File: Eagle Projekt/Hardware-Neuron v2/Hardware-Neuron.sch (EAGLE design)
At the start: 58 parts, among them IC1 74LVC1G125DBV, IC10 74LVC1G125DBV, IC11 74LVC1G125DBV, IC12 74LVC1G125DBV, IC13 74AHC1G86DBV, IC14 74LVC1G125DBV, IC15 74LVC1G125DBV, IC16 74LVC1G125DBV, IC17 74LVC1G125DBV, IC18 74AHC1G14DCK, IC19 74LVC1G125DBV, IC2 74LVC1G125DBV, IC20 74LVC1G125DBV, IC21 74LVC1G125DBV, IC22 74LVC1G125DBV, IC3 74LVC1G125DBV, IC4 74LVC1G125DBV, IC5 74LVC1G125DBV, IC6 74LVC1G125DBV, IC7 74AUC1G06DBV, IC8 74AHC1G08DBV, IC9 74LVC1G125DBV, Q1 FDN360P, Q10 FDN360P, Q11 BSS123, Q2 FDN360P, Q3 FDN360P, Q4 FDN360P, Q5 FDN360P, Q6 FDN360P, Q7 FDN360P, Q8 FDN360P, Q9 FDN360P

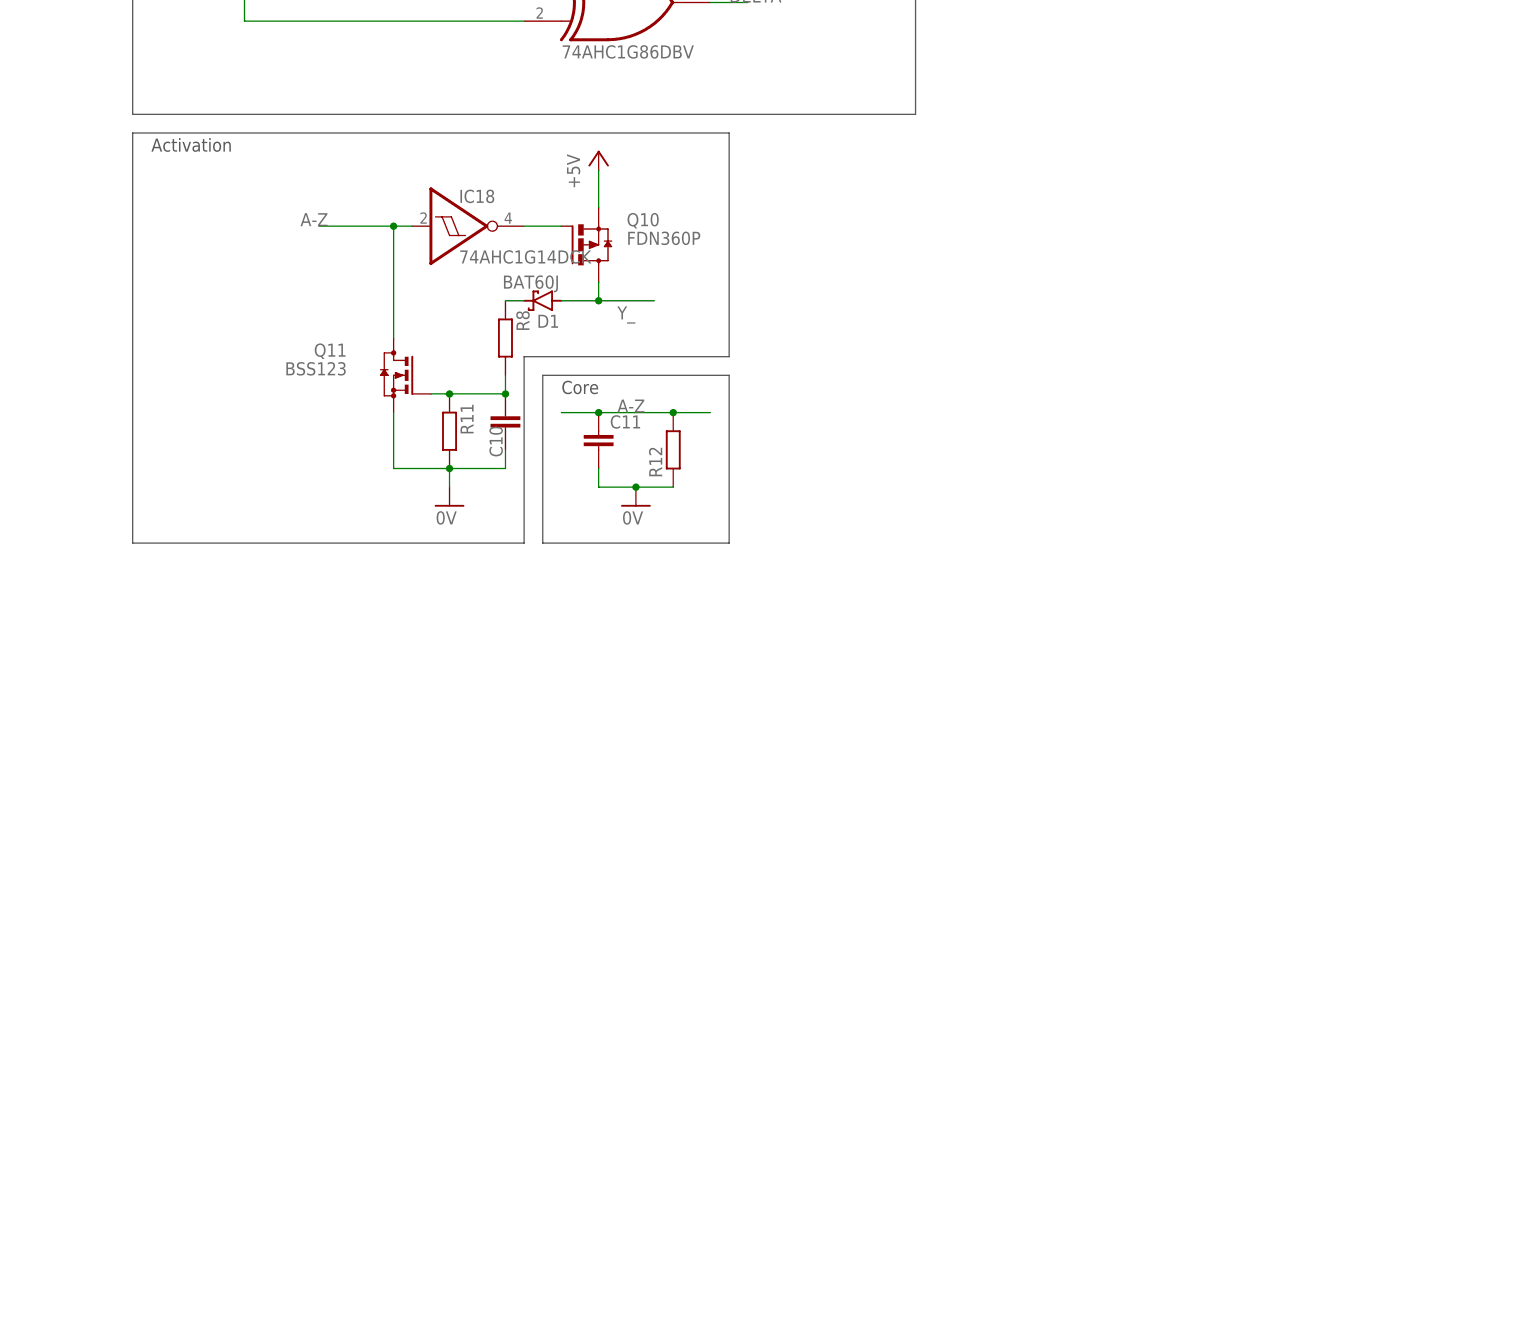
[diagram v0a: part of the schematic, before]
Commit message: malik aar und eagle
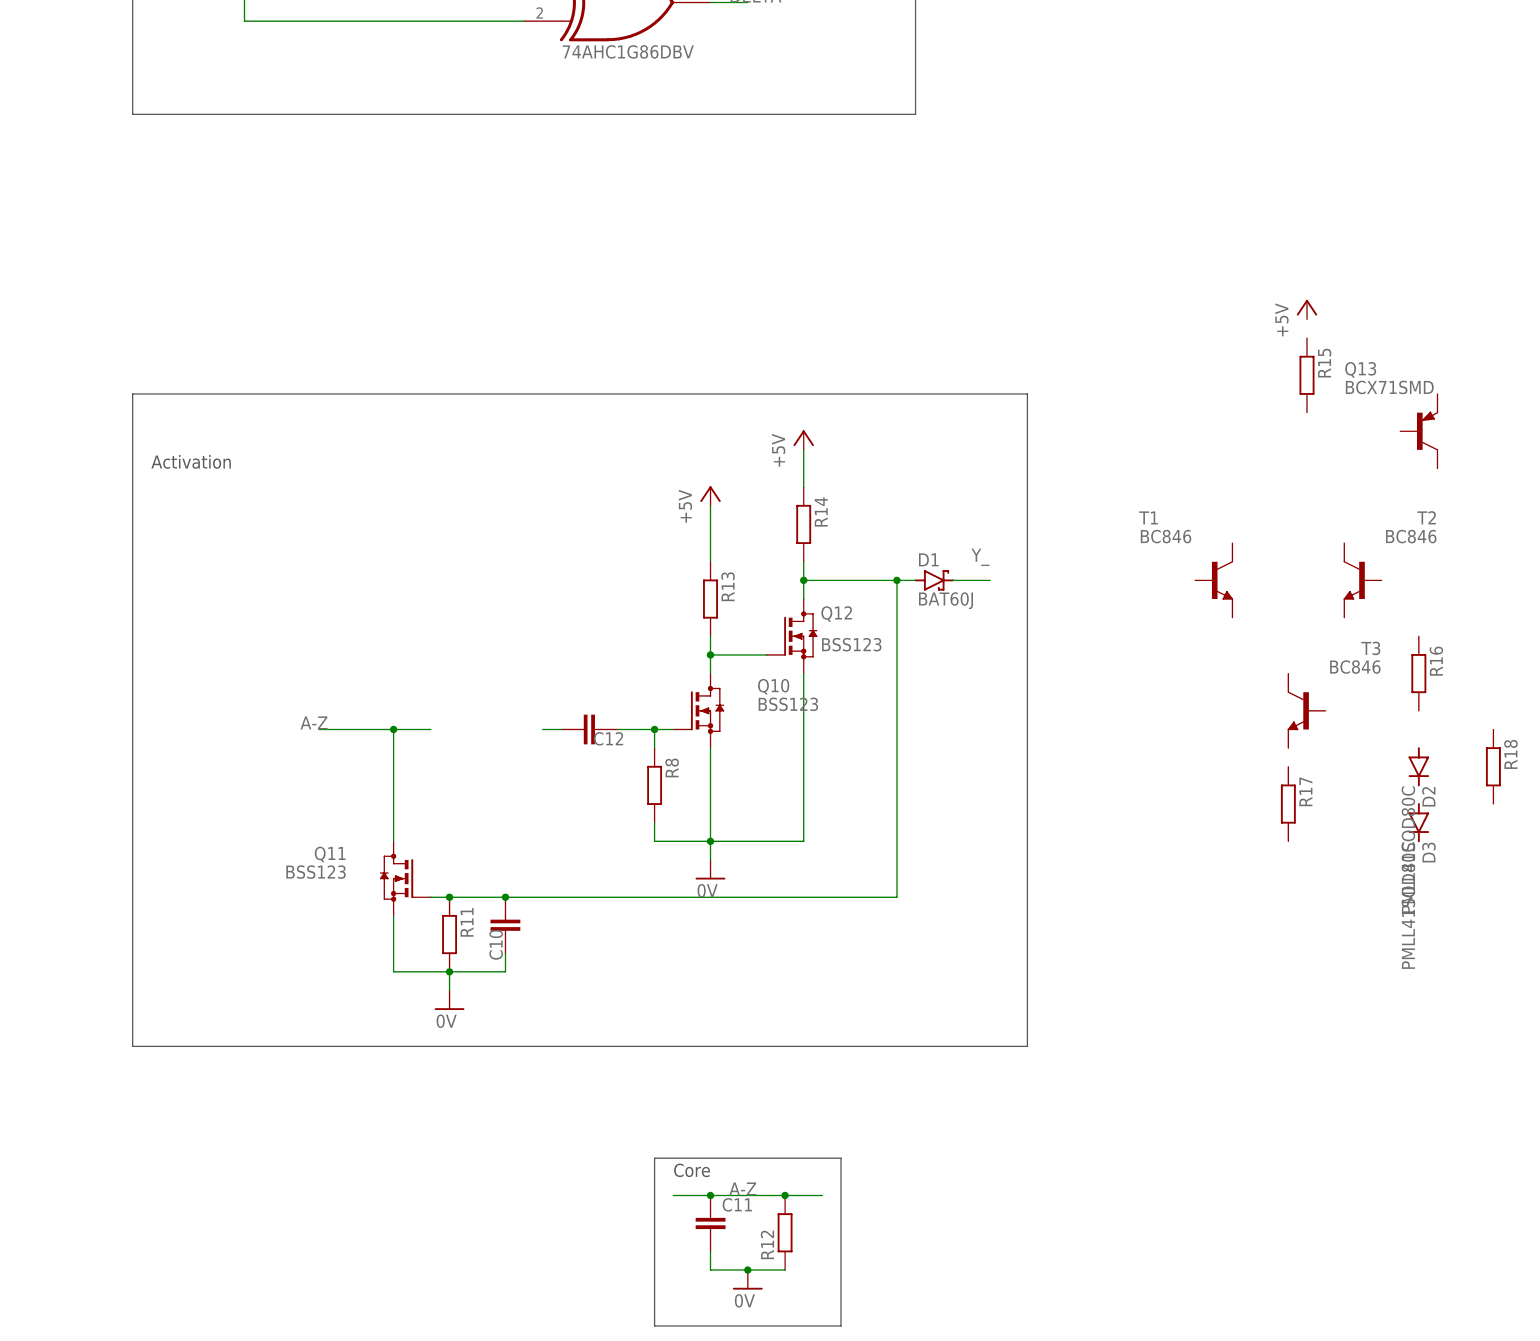
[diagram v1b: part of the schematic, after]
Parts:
- removed IC18: 74AHC1G14DCK, 74xx-little-de:74AHC1G14DCK
- added C12: (no value), rcl:C-EUC1206
- added D2, D3: PMLL41SOD80C, diode:PMLL41SOD80C
- added Q12: BSS123, transistor-small-signal:BSS123
- added Q13: BCX71SMD, transistor-pnp:BCX71SMD
- added R13, R14, R15, R16, R17, R18: (no value), rcl:R-EU_R1206
- added T1, T2, T3: BC846, transistor:BC846
- Q10: value FDN360P -> BSS123; device transistor-power:FDN360P -> transistor-small-signal:BSS123
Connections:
- new net N$3: C12.2, Q10.G, R8.1
- net +5V: now also R13.1, R14.1; no longer Q10.S
- net 0V: now also Q10.S, Q12.S, R8.2
- net A-Z: no longer IC18A.I
- net N$4: now also D1.A, Q12.D, R14.2; no longer R8.2
- net N$5: now also Q10.D, Q12.G, R13.2; no longer D1.C, R8.1
- net N$7: now also C12.1; no longer IC18A.O, Q10.G
- net Y_: now also D1.C; no longer D1.A, Q10.D
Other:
- moved on the sheet: C10, C11, D1, Q11, R11, R12, R8
